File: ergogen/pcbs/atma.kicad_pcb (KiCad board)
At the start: 2 copper layers, 114.3 x 82.4 mm, 61 parts

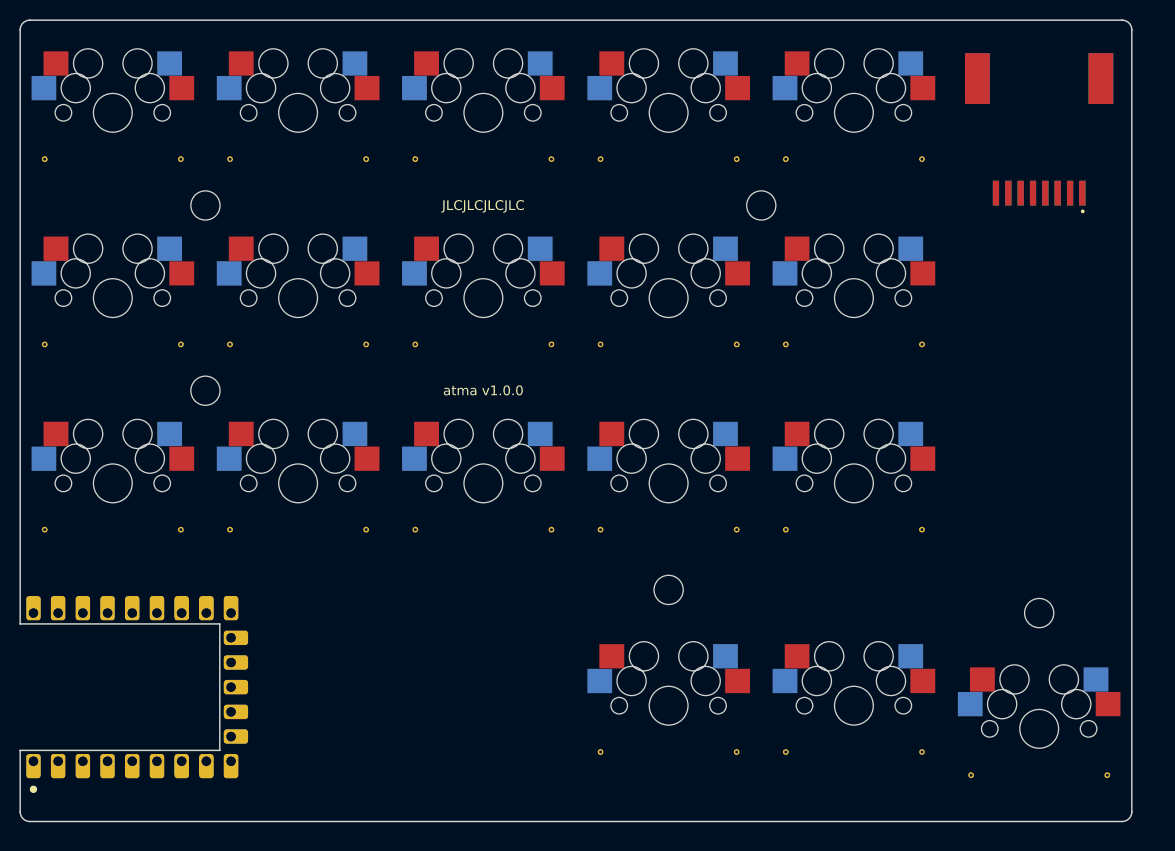
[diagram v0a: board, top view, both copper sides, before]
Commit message: better case idea
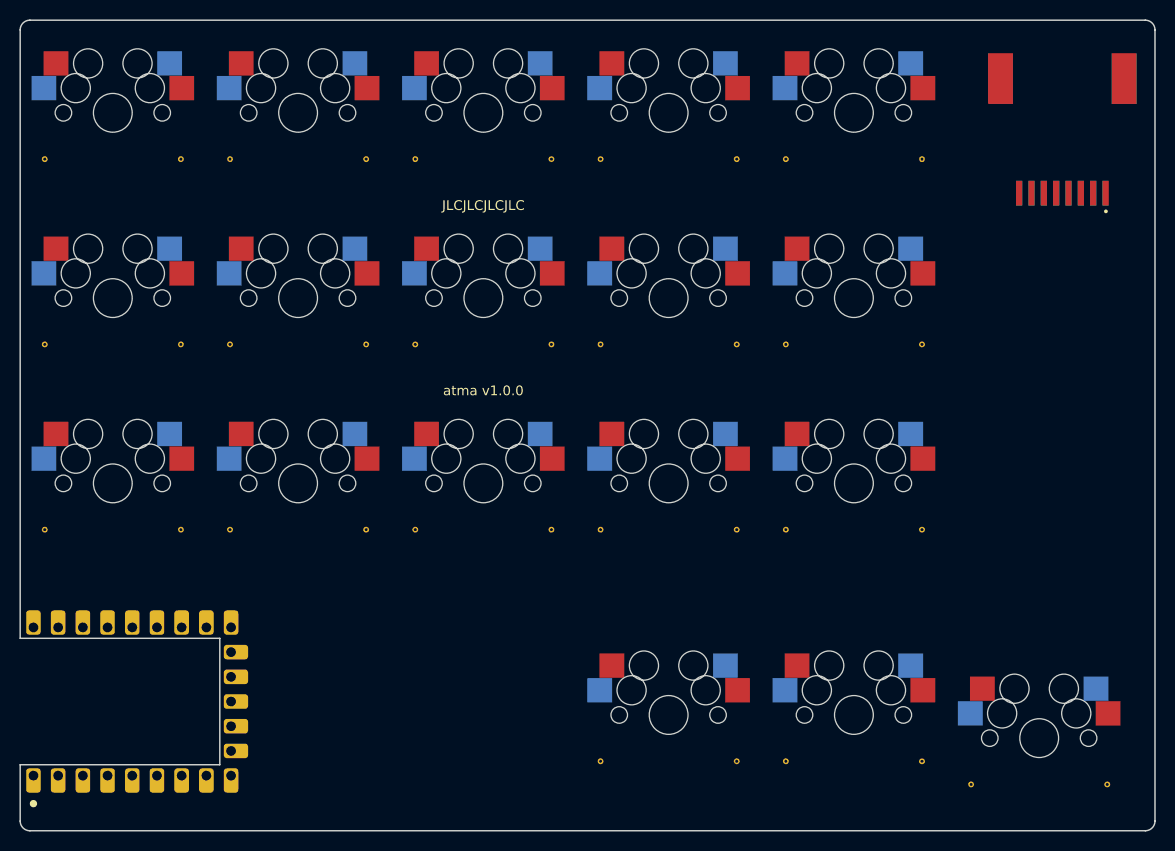
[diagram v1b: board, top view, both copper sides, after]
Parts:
- removed the ? at (209.6, 163.4)
- removed the ? at (247.7, 165.7)
- removed the ? at (161.9, 123.8)
- removed the ? at (161.9, 142.9)
- removed the ? at (219.1, 123.8)
- removed the REF** at (202.6, 180.0)
- removed the REF** at (221.6, 180.0)
- removed the REF** at (240.7, 182.4)
- removed the REF** at (216.6, 180.0)
- removed the REF** at (235.6, 180.0)
- removed the REF** at (254.7, 182.4)
- added REF**: VIA-0.6mm, VIA-0.6mm, F.Cu at (202.6, 181.0)
- added REF**: VIA-0.6mm, VIA-0.6mm, F.Cu at (221.6, 181.0)
- added REF**: VIA-0.6mm, VIA-0.6mm, F.Cu at (240.7, 183.4)
- added REF**: VIA-0.6mm, VIA-0.6mm, F.Cu at (216.6, 181.0)
- added REF**: VIA-0.6mm, VIA-0.6mm, F.Cu at (235.6, 181.0)
- added REF**: VIA-0.6mm, VIA-0.6mm, F.Cu at (254.7, 183.4)
- moved ? 2.38 mm to (250.0, 121.7)
- moved ? 1.48 mm to (154.4, 174.8)
- moved S16 0.95 mm to (209.6, 176.2)
- moved S17 0.95 mm to (228.6, 176.2)
- moved S18 0.95 mm to (247.7, 178.6)
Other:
- board size 114.3 x 82.4 mm -> 116.7 x 83.3 mm
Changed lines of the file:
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@@
   )
     (module rp2040_zero_tht_pads (layer F.Cu)
-      (at 154.4 173.35500000000002 90)
+      (at 154.4 174.83125 90)
       (attr through_hole)
         (pad 1 thru_hole roundrect (at 7.62 -10.16 270) (size 2.5 1.5) (drill 1 (offset -0.5 0)) (layers *.Cu *.Mask) (roundrect_rratio 0.2) (net 1 "matrix_pinky_bottom"))
@@
       )
     (module "44144-0003" (layer F.Cu)
-      (at 247.65000000000003 121.7295 180)
+      (at 250.03125000000003 121.7295 180)
       (fp_line (start -7.62 0) (end 7.62 0) (layer F.Fab) (width 0.2))
       (fp_line (start 7.62 0) (end 7.62 16.89) (layer F.Fab) (width 0.2))
@@
         )
       (module MX (layer F.Cu)
-      (at 209.55 175.26 0)
+      (at 209.55 176.2125 0)
       (fp_text reference "S16" (at 0 0) (layer F.SilkS) hide (effects (font (size 1.27 1.27) (thickness 0.15))))
       (fp_text value "" (at 0 0) (layer F.SilkS) hide (effects (font (size 1.27 1.27) (thickness 0.15))))
@@
         )
       (module MX (layer F.Cu)
-      (at 228.60000000000002 175.26 0)
+      (at 228.60000000000002 176.2125 0)
       (fp_text reference "S17" (at 0 0) (layer F.SilkS) hide (effects (font (size 1.27 1.27) (thickness 0.15))))
       (fp_text value "" (at 0 0) (layer F.SilkS) hide (effects (font (size 1.27 1.27) (thickness 0.15))))
@@
         )
       (module MX (layer F.Cu)
-      (at 247.65 177.64124999999999 0)
+      (at 247.65 178.59375 0)
       (fp_text reference "S18" (at 0 0) (layer F.SilkS) hide (effects (font (size 1.27 1.27) (thickness 0.15))))
       (fp_text value "" (at 0 0) (layer F.SilkS) hide (effects (font (size 1.27 1.27) (thickness 0.15))))
@@
       )
       (module VIA-0.6mm (layer F.Cu)
-      (at 202.55 180.02249999999998 0)
+      (at 202.55 180.975 0)
       (fp_text reference REF** (at 0 1.4) (layer F.SilkS) hide (effects (font (size 1 1) (thickness 0.15))))
       (fp_text value VIA-0.6mm (at 0 -1.4) (layer F.Fab) hide (effects (font (size 1 1) (thickness 0.15))))
@@
       )
       (module VIA-0.6mm (layer F.Cu)
-      (at 221.60000000000002 180.02249999999998 0)
+      (at 221.60000000000002 180.975 0)
       (fp_text reference REF** (at 0 1.4) (layer F.SilkS) hide (effects (font (size 1 1) (thickness 0.15))))
       (fp_text value VIA-0.6mm (at 0 -1.4) (layer F.Fab) hide (effects (font (size 1 1) (thickness 0.15))))
@@
       )
       (module VIA-0.6mm (layer F.Cu)
-      (at 240.65 182.40374999999997 0)
+      (at 240.65 183.35625 0)
       (fp_text reference REF** (at 0 1.4) (layer F.SilkS) hide (effects (font (size 1 1) (thickness 0.15))))
       (fp_text value VIA-0.6mm (at 0 -1.4) (layer F.Fab) hide (effects (font (size 1 1) (thickness 0.15))))
@@
       )
       (module VIA-0.6mm (layer F.Cu)
-      (at 216.55 180.02249999999998 0)
+      (at 216.55 180.975 0)
       (fp_text reference REF** (at 0 1.4) (layer F.SilkS) hide (effects (font (size 1 1) (thickness 0.15))))
       (fp_text value VIA-0.6mm (at 0 -1.4) (layer F.Fab) hide (effects (font (size 1 1) (thickness 0.15))))
@@
       )
       (module VIA-0.6mm (layer F.Cu)
-      (at 235.60000000000002 180.02249999999998 0)
+      (at 235.60000000000002 180.975 0)
       (fp_text reference REF** (at 0 1.4) (layer F.SilkS) hide (effects (font (size 1 1) (thickness 0.15))))
       (fp_text value VIA-0.6mm (at 0 -1.4) (layer F.Fab) hide (effects (font (size 1 1) (thickness 0.15))))
@@
       )
       (module VIA-0.6mm (layer F.Cu)
-      (at 254.65 182.40374999999997 0)
+      (at 254.65 183.35625 0)
       (fp_text reference REF** (at 0 1.4) (layer F.SilkS) hide (effects (font (size 1 1) (thickness 0.15))))
       (fp_text value VIA-0.6mm (at 0 -1.4) (layer F.Fab) hide (effects (font (size 1 1) (thickness 0.15))))
@@
                 (effects (font (size 1 1) (thickness 0.15)) )
             )
-      (module DrillHole (layer "F.Cu")
-      (at 209.55 163.35375 0)
-      (pad "" np_thru_hole circle (at 0 0) (size 3 3) (drill 3) (layers *.Cu *.Mask))
-    )
-      (module DrillHole (layer "F.Cu")
-      (at 247.65 165.73499999999999 0)
-      (pad "" np_thru_hole circle (at 0 0) (size 3 3) (drill 3) (layers *.Cu *.Mask))
-    )
-      (module DrillHole (layer "F.Cu")
-      (at 161.925 123.82499999999999 0)
-      (pad "" np_thru_hole circle (at 0 0) (size 3 3) (drill 3) (layers *.Cu *.Mask))
-    )
-      (module DrillHole (layer "F.Cu")
-      (at 161.925 142.875 0)
-      (pad "" np_thru_hole circle (at 0 0) (size 3 3) (drill 3) (layers *.Cu *.Mask))
-    )
-      (module DrillHole (layer "F.Cu")
-      (at 219.07500000000002 123.82499999999999 0)
-      (pad "" np_thru_hole circle (at 0 0) (size 3 3) (drill 3) (layers *.Cu *.Mask))
-    )
-            (gr_line (start 142.875 186.16625) (end 142.875 179.85500000000002) (angle 90) (layer Edge.Cuts) (width 0.15))
-(gr_line (start 142.875 166.85500000000002) (end 142.875 105.77499999999999) (angle 90) (layer Edge.Cuts) (width 0.15))
-(gr_line (start 143.875 104.77499999999999) (end 256.175 104.77499999999999) (angle 90) (layer Edge.Cuts) (width 0.15))
-(gr_line (start 257.175 105.77499999999999) (end 257.175 186.16625) (angle 90) (layer Edge.Cuts) (width 0.15))
-(gr_line (start 256.175 187.16625) (end 143.875 187.16625) (angle 90) (layer Edge.Cuts) (width 0.15))
+            (gr_line (start 142.875 187.11875) (end 142.875 181.33125) (angle 90) (layer Edge.Cuts) (width 0.15))
+(gr_line (start 142.875 168.33125) (end 142.875 105.77499999999999) (angle 90) (layer Edge.Cuts) (width 0.15))
+(gr_line (start 143.875 104.77499999999999) (end 258.55625000000003 104.77499999999999) (angle 90) (layer Edge.Cuts) (width 0.15))
+(gr_line (start 259.55625000000003 105.77499999999999) (end 259.55625000000003 187.11875) (angle 90) (layer Edge.Cuts) (width 0.15))
+(gr_line (start 258.55625000000003 188.11875) (end 143.875 188.11875) (angle 90) (layer Edge.Cuts) (width 0.15))
 (gr_arc (start 143.875 105.77499999999999) (end 143.875 104.77499999999999) (angle -90) (layer Edge.Cuts) (width 0.15))
-(gr_arc (start 256.175 105.77499999999999) (end 257.175 105.77499999999999) (angle -90) (layer Edge.Cuts) (width 0.15))
-(gr_arc (start 256.175 186.16625) (end 256.175 187.16625) (angle -90) (layer Edge.Cuts) (width 0.15))
-(gr_arc (start 143.875 186.16625) (end 142.875 186.16625) (angle -90) (layer Edge.Cuts) (width 0.15))
-(gr_line (start 142.875 179.85500000000002) (end 163.4 179.85500000000002) (angle 90) (layer Edge.Cuts) (width 0.15))
-(gr_line (start 163.4 179.85500000000002) (end 163.4 166.85500000000002) (angle 90) (layer Edge.Cuts) (width 0.15))
-(gr_line (start 163.4 166.85500000000002) (end 142.875 166.85500000000002) (angle 90) (layer Edge.Cuts) (width 0.15))
+(gr_arc (start 258.55625000000003 105.77499999999999) (end 259.55625000000003 105.77499999999999) (angle -90) (layer Edge.Cuts) (width 0.15))
+(gr_arc (start 258.55625000000003 187.11875) (end 258.55625000000003 188.11875) (angle -90) (layer Edge.Cuts) (width 0.15))
+(gr_arc (start 143.875 187.11875) (end 142.875 187.11875) (angle -90) (layer Edge.Cuts) (width 0.15))
+(gr_line (start 142.875 181.33125) (end 163.4 181.33125) (angle 90) (layer Edge.Cuts) (width 0.15))
+(gr_line (start 163.4 181.33125) (end 163.4 168.33125) (angle 90) (layer Edge.Cuts) (width 0.15))
+(gr_line (start 163.4 168.33125) (end 142.875 168.33125) (angle 90) (layer Edge.Cuts) (width 0.15))
 )
